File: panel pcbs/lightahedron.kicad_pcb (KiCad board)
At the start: 2 copper layers, 68.3 x 59.3 mm, 60 parts, among them J1 CONN, M1 Magnet 5x2mm, M2 Magnet 5x2mm, M3 Magnet 5x2mm

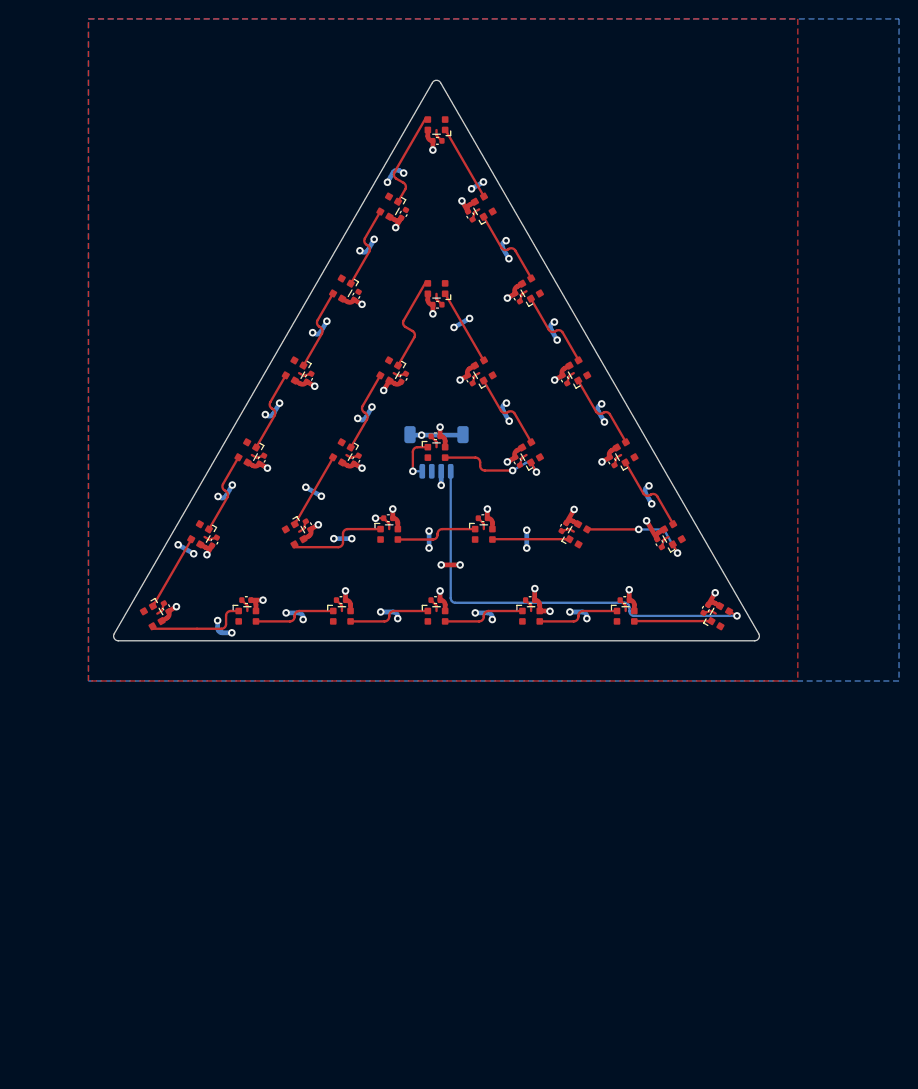
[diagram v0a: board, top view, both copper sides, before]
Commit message: cleanup, work on pcbs, finish frame, add render
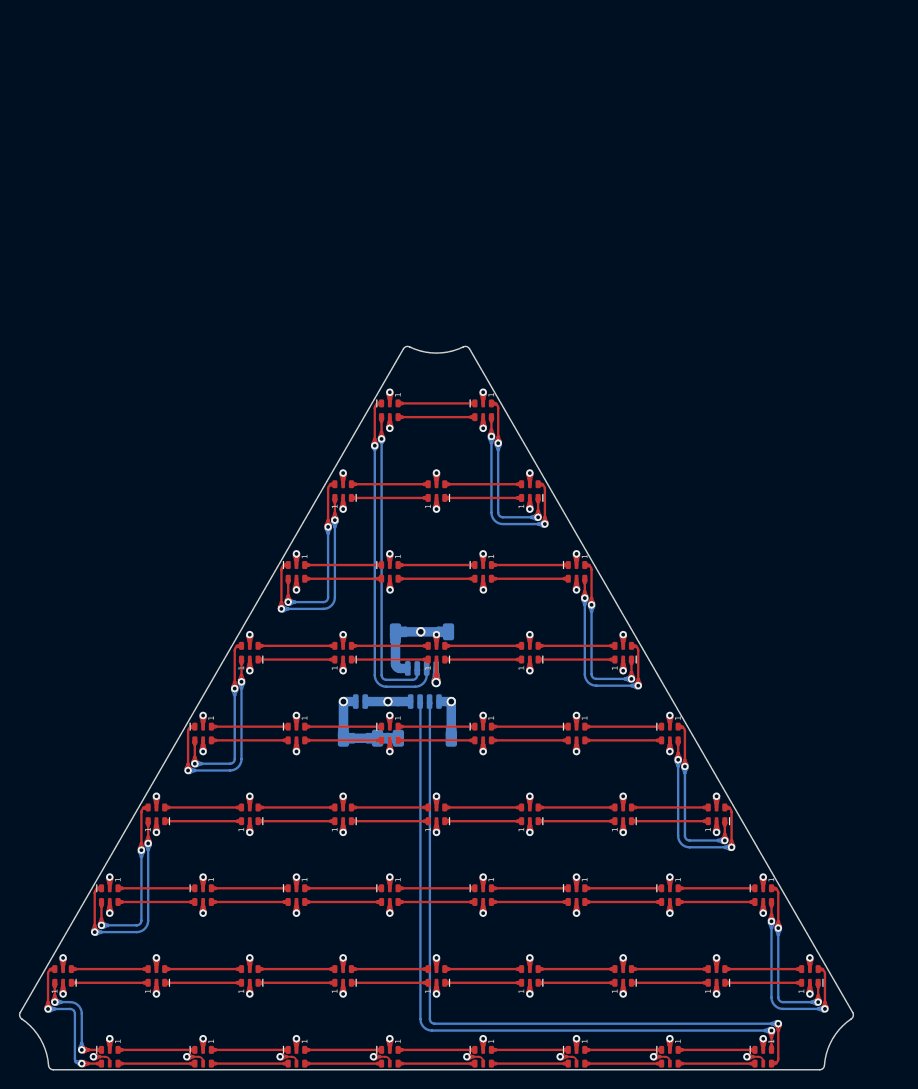
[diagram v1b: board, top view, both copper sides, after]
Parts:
- removed C1, C10, C11, C12, C13, C14, C15, C16, C17, C18, C19, C2, C20, C21, C22, C23, C24, C25, C26, C27, C28, C3, C4, C5, C6, C7, C8, C9: 100nf, Capacitor_SMD:C_0402_1005Metric
- removed L1, L10, L11, L12, L13, L14, L15, L16, L17, L18, L19, L2, L20, L21, L22, L23, L24, L25, L26, L27, L28, L3, L4, L5, L6, L7, L8, L9: WS2812_2020, marbastlib-various:LED_WS2812_2020
- added D1: SK9822-EC20, custom:sk9822-2020, F.Cu at (-4.93, -4.45)
- added D10: SK9822-EC20, custom:sk9822-2020, F.Cu at (-19.7, 21.2)
- added D11: SK9822-EC20, custom:sk9822-2020, F.Cu at (-9.87, 21.2)
- added D12: SK9822-EC20, custom:sk9822-2020, F.Cu at (-0.00, 21.2)
- added D13: SK9822-EC20, custom:sk9822-2020, F.Cu at (9.87, 21.2)
- added D14: SK9822-EC20, custom:sk9822-2020, F.Cu at (19.7, 21.2)
- added D15: SK9822-EC20, custom:sk9822-2020, F.Cu at (-24.7, 29.7)
- added D16: SK9822-EC20, custom:sk9822-2020, F.Cu at (-14.8, 29.7)
- added D17: SK9822-EC20, custom:sk9822-2020, F.Cu at (-4.94, 29.7)
- added D18: SK9822-EC20, custom:sk9822-2020, F.Cu at (4.94, 29.7)
- added D19: SK9822-EC20, custom:sk9822-2020, F.Cu at (14.8, 29.7)
- added D2: SK9822-EC20, custom:sk9822-2020, F.Cu at (4.93, -4.45)
- added D20: SK9822-EC20, custom:sk9822-2020, F.Cu at (24.7, 29.7)
- added D21: SK9822-EC20, custom:sk9822-2020, F.Cu at (-29.6, 38.3)
- added D22: SK9822-EC20, custom:sk9822-2020, F.Cu at (-19.7, 38.3)
- added D23: SK9822-EC20, custom:sk9822-2020, F.Cu at (-9.87, 38.3)
- added D24: SK9822-EC20, custom:sk9822-2020, F.Cu at (0.00, 38.3)
- added D25: SK9822-EC20, custom:sk9822-2020, F.Cu at (9.87, 38.3)
- added D26: SK9822-EC20, custom:sk9822-2020, F.Cu at (19.7, 38.3)
- added D27: SK9822-EC20, custom:sk9822-2020, F.Cu at (29.6, 38.3)
- added D28: SK9822-EC20, custom:sk9822-2020, F.Cu at (-34.5, 46.8)
- added D29: SK9822-EC20, custom:sk9822-2020, F.Cu at (-24.7, 46.8)
- added D3: SK9822-EC20, custom:sk9822-2020, F.Cu at (-9.87, 4.09)
- added D30: SK9822-EC20, custom:sk9822-2020, F.Cu at (-14.8, 46.8)
- added D31: SK9822-EC20, custom:sk9822-2020, F.Cu at (-4.94, 46.8)
- added D32: SK9822-EC20, custom:sk9822-2020, F.Cu at (4.93, 46.8)
- added D33: SK9822-EC20, custom:sk9822-2020, F.Cu at (14.8, 46.8)
- added D34: SK9822-EC20, custom:sk9822-2020, F.Cu at (24.7, 46.8)
- added D35: SK9822-EC20, custom:sk9822-2020, F.Cu at (34.5, 46.8)
- added D36: SK9822-EC20, custom:sk9822-2020, F.Cu at (-39.5, 55.4)
- added D37: SK9822-EC20, custom:sk9822-2020, F.Cu at (-29.6, 55.4)
- added D38: SK9822-EC20, custom:sk9822-2020, F.Cu at (-19.7, 55.4)
- added D39: SK9822-EC20, custom:sk9822-2020, F.Cu at (-9.87, 55.4)
- added D4: SK9822-EC20, custom:sk9822-2020, F.Cu at (0.00, 4.09)
- added D40: SK9822-EC20, custom:sk9822-2020, F.Cu at (-0.00, 55.4)
- added D41: SK9822-EC20, custom:sk9822-2020, F.Cu at (9.87, 55.4)
- added D42: SK9822-EC20, custom:sk9822-2020, F.Cu at (19.7, 55.4)
- added D43: SK9822-EC20, custom:sk9822-2020, F.Cu at (29.6, 55.4)
- added D44: SK9822-EC20, custom:sk9822-2020, F.Cu at (39.5, 55.4)
- added D45: SK9822-EC20, custom:sk9822-2020, F.Cu at (-34.5, 63.9)
- added D46: SK9822-EC20, custom:sk9822-2020, F.Cu at (-24.7, 63.9)
- added D47: SK9822-EC20, custom:sk9822-2020, F.Cu at (-14.8, 63.9)
- added D48: SK9822-EC20, custom:sk9822-2020, F.Cu at (-4.94, 63.9)
- added D49: SK9822-EC20, custom:sk9822-2020, F.Cu at (4.93, 63.9)
- added D5: SK9822-EC20, custom:sk9822-2020, F.Cu at (9.87, 4.09)
- added D50: SK9822-EC20, custom:sk9822-2020, F.Cu at (14.8, 63.9)
- added D51: SK9822-EC20, custom:sk9822-2020, F.Cu at (24.7, 63.9)
- added D52: SK9822-EC20, custom:sk9822-2020, F.Cu at (34.5, 63.9)
- added D6: SK9822-EC20, custom:sk9822-2020, F.Cu at (-14.8, 12.6)
- added D7: SK9822-EC20, custom:sk9822-2020, F.Cu at (-4.93, 12.6)
- added D8: SK9822-EC20, custom:sk9822-2020, F.Cu at (4.93, 12.6)
- added D9: SK9822-EC20, custom:sk9822-2020, F.Cu at (14.8, 12.6)
- added J2: OUT, Connector_JST:JST_SH_SM04B-SRSS-TB_1x04-1MP_P1.00mm_Horizontal, B.Cu at (-1.24, 28.3)
- added J3: POWER, Connector_JST:JST_SH_SM02B-SRSS-TB_1x02-1MP_P1.00mm_Horizontal, B.Cu at (-8.04, 28.3)
- J1: value CONN -> IN
- M1, M2, M3: value Magnet 5x2mm -> Magnet 5x1mm; footprint magnets:Magnet_D5mm_L2mm -> custom:Magnet_D5mm_L2mm
- moved M1 87.2 mm to (-32.8, 56.8)
- moved M3 43.6 mm to (32.8, 56.8), turned to 180 degrees
- moved M2 24.1 mm to (0.00, 0.00), turned to 180 degrees
- moved J1 20.9 mm to (-1.54, 20.8)
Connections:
- J1 pad 1: RGB_OUT -> GND
- J1 pad 2: VCC -> CIN
- J1 pad 3: GND -> DIN
- J1 pad 4: RGB_IN -> VCC
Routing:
- net GND: track 93.4 -> 642.3 mm, vias 49 -> 55
- net VCC: track 75.1 -> 595.3 mm, vias 31 -> 53
- net COUT: track 0.00 -> 75.3 mm, vias 0 -> 1
- net DOUT: track 0.00 -> 73.4 mm, vias 0 -> 1
- net RGB_IN: track 45.8 -> 0.00 mm, vias 1 -> 0
- net DIN: track 0.00 -> 36.7 mm, vias 0 -> 1
- net CIN: track 0.00 -> 32.3 mm, vias 0 -> 1
- net D6: track 0.00 -> 21.9 mm, vias 0 -> 2
- net D4: track 0.00 -> 21.9 mm, vias 0 -> 2
- net D2: track 0.00 -> 21.9 mm, vias 0 -> 2
- net C5: track 0.00 -> 21.1 mm, vias 0 -> 2
- net C7: track 0.00 -> 21.1 mm, vias 0 -> 2
- net C1: track 0.00 -> 21.1 mm, vias 0 -> 2
- net C3: track 0.00 -> 21.1 mm, vias 0 -> 2
- net C6: track 0.00 -> 19.7 mm, vias 0 -> 2
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- removed copper zone on F.Cu, net GND
- removed copper zone on B.Cu, net VCC
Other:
- board size 68.3 x 59.3 mm -> 88.2 x 76.5 mm
- copper layers 2 -> 4
